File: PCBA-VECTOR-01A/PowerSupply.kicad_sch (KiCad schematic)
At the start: 61 parts, among them J3 Conn_02x04_Odd_Even, U1 TPS62913, U3 LM5013DDAR, U4 TL1963ADCQR, U5 TPS7A2033PDQNR

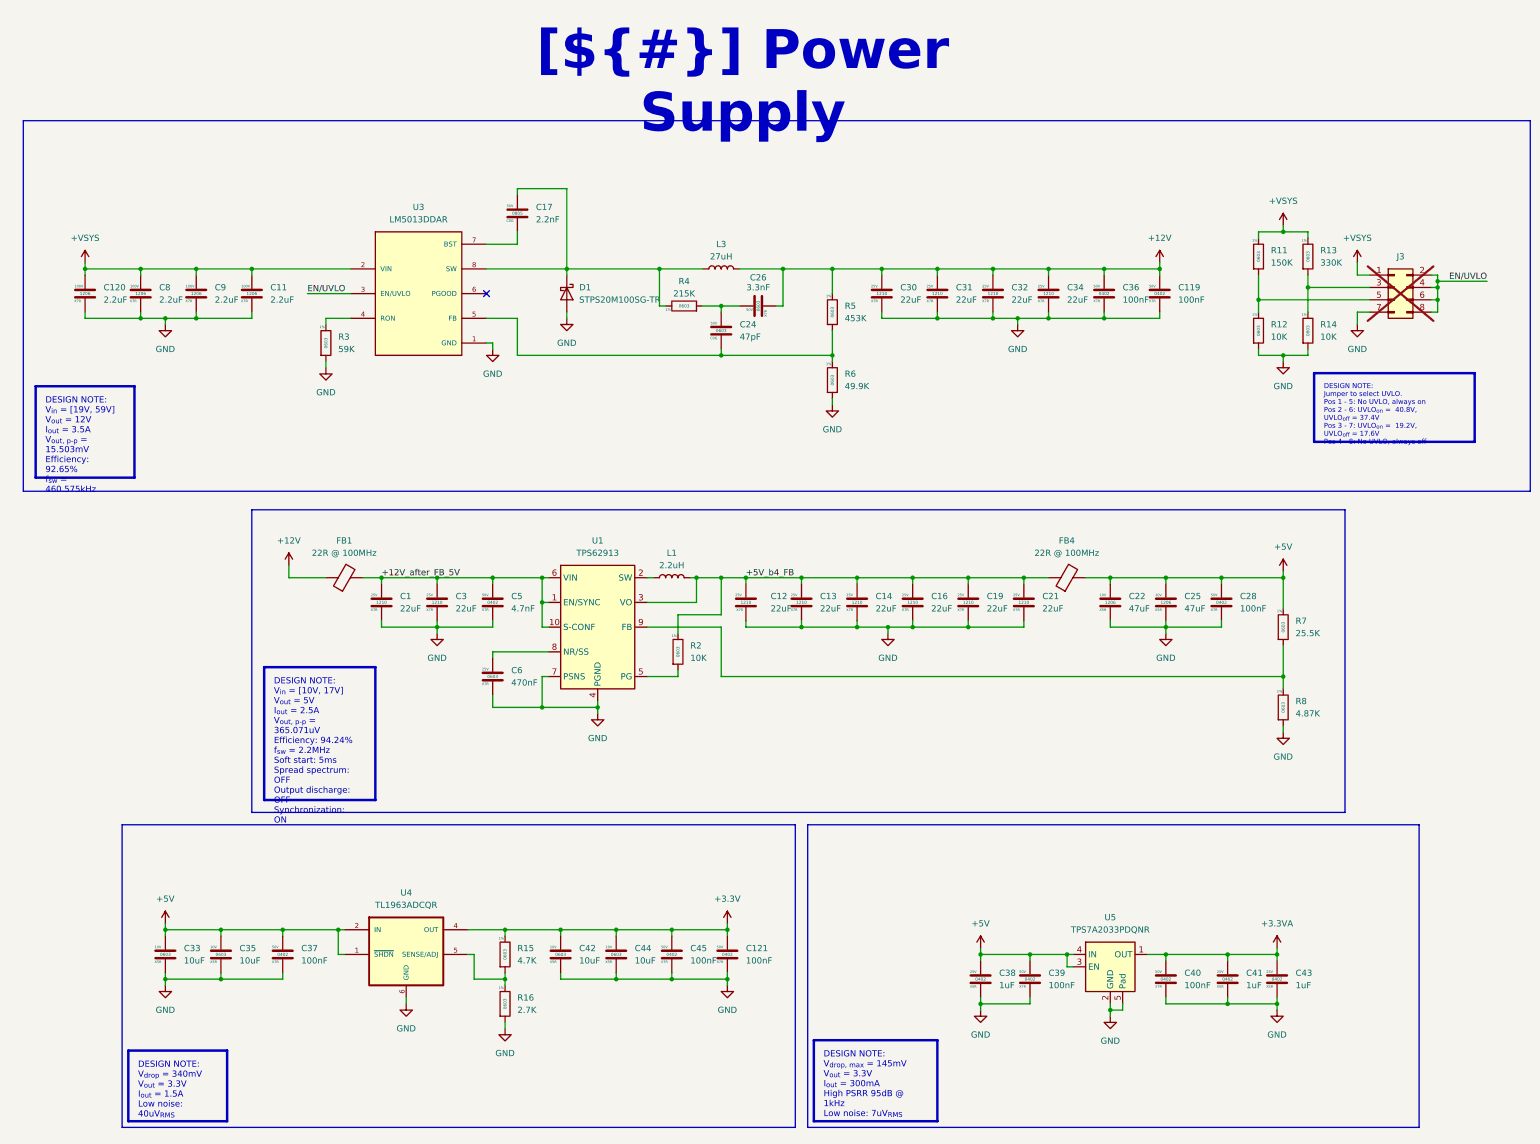
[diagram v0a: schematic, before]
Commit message: Finished schematic?
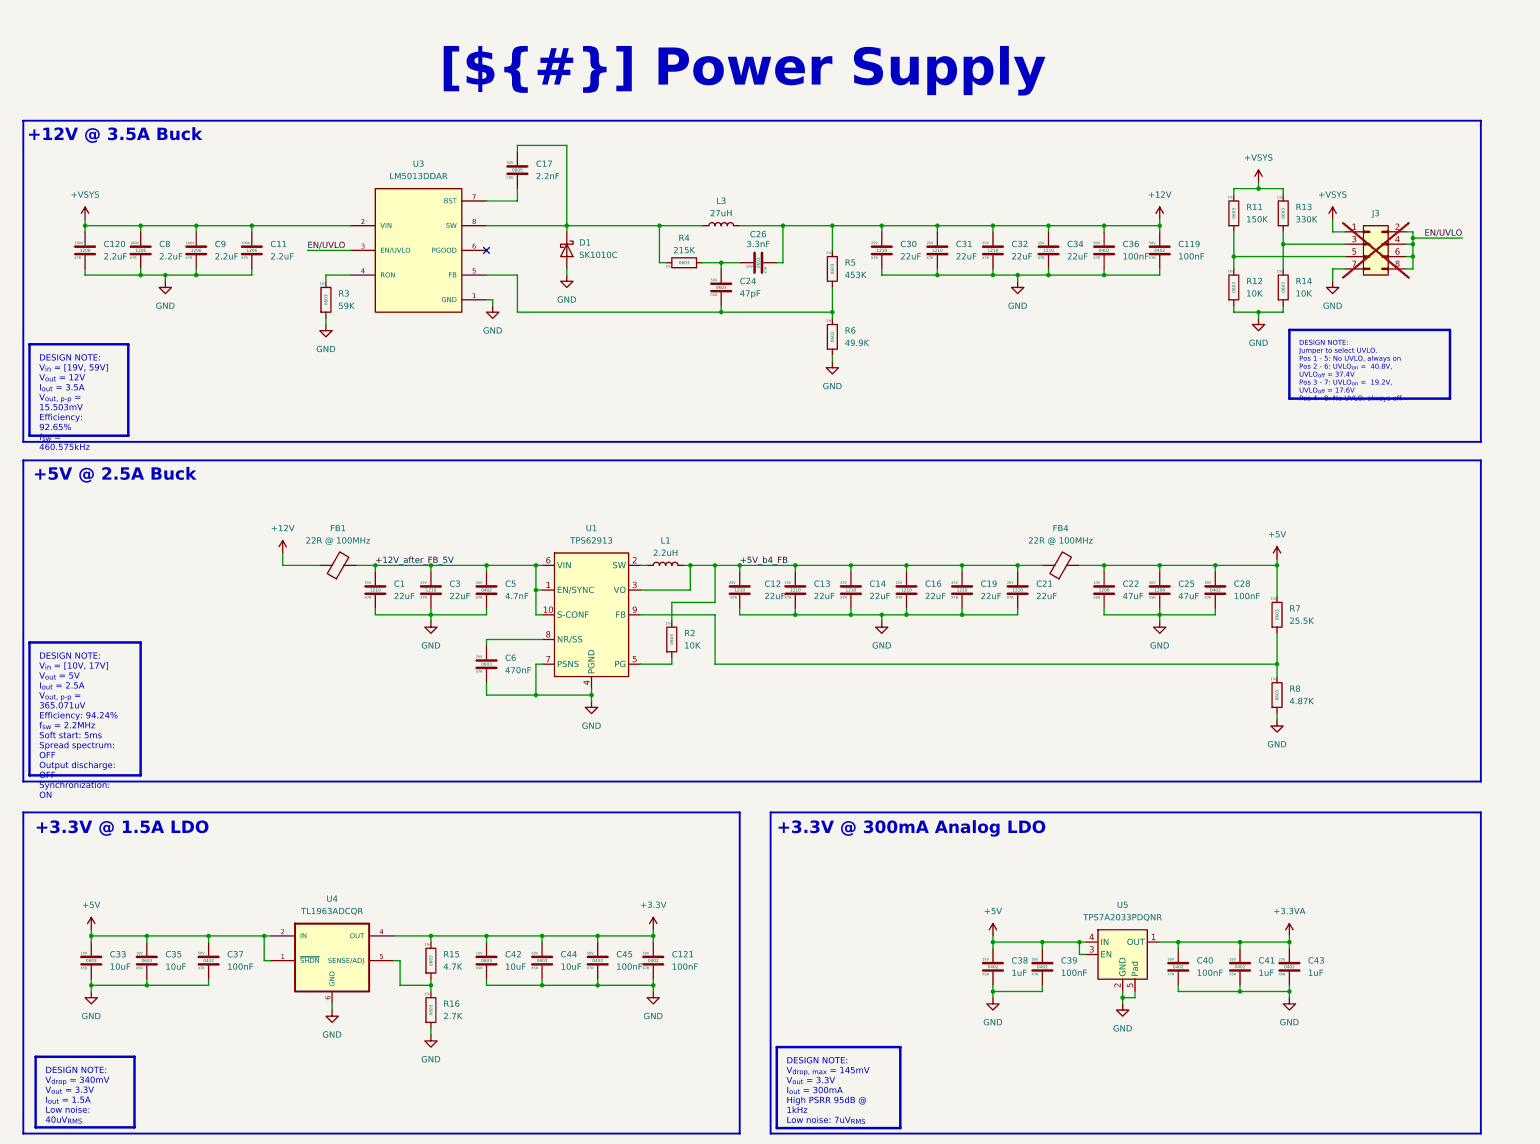
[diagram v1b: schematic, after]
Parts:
- removed D1: STPS20M100SG-TR, Package_TO_SOT_SMD:TO-263-2, symbol Device:D_Schottky
- added D1: SK1010C, Diode_SMD:D_SMC, symbol Synapse:D_Schottky
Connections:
- net GND: now also D1.2 (A)
- net at C17.1, L3.1, R4.1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: now also D1.1 (K)
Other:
- note added: "+12V @ 3.5A Buck"
- note added: "+3.3V @ 1.5A LDO"
- note added: "+3.3V @ 300mA Analog LDO"
- note added: "+5V @ 2.5A Buck"
- moved on the sheet: C1, C11, C119, C12, C120, C121, C13, C14, C16, C17, C19, C21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
